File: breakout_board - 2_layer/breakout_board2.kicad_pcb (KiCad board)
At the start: 2 copper layers, 54 parts, among them J1 Conn_01x14, J2 Conn_01x14, J3 CONN_01X03, J4 CONN_02x04, J5 Conn_01x04, U1 TB6612FNG, U2 LP5907SNX-3.3/NOPB, U3 LSF0204RUTR, U4 ADP3330, U5 TLV70718PDQNR

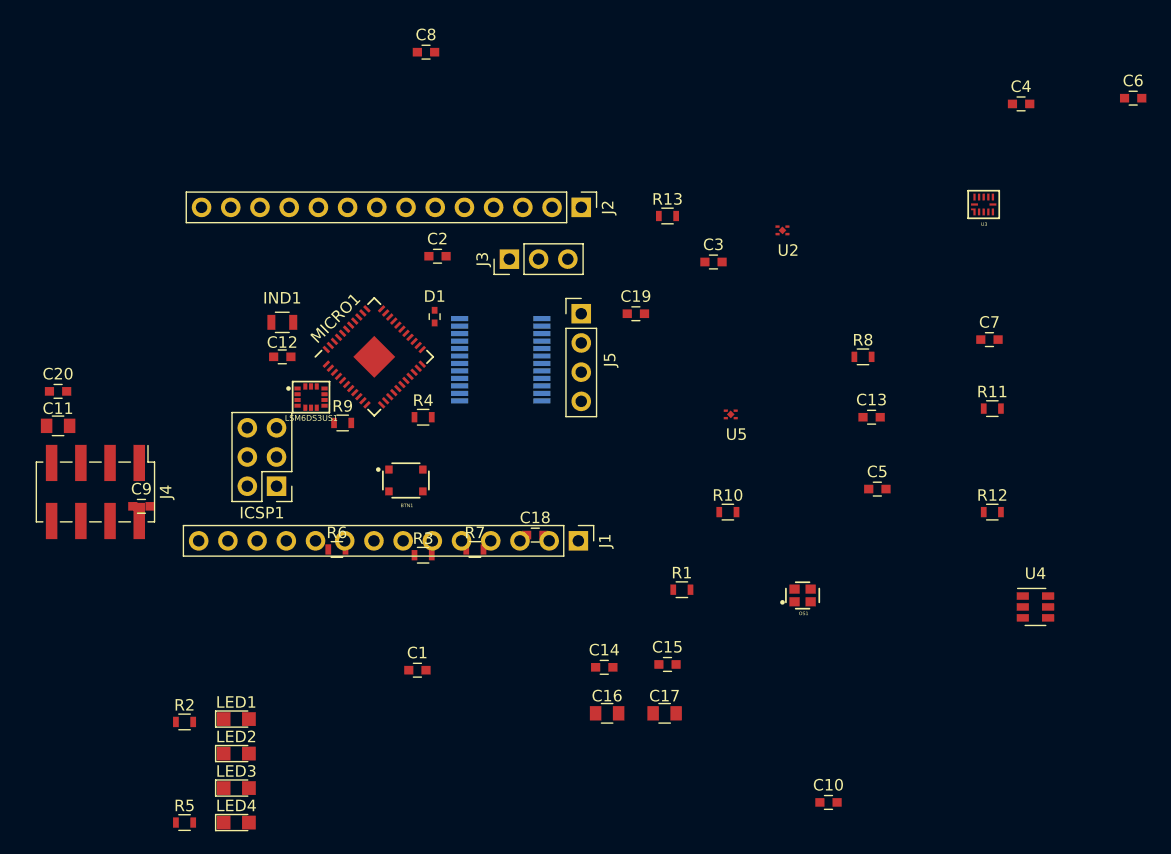
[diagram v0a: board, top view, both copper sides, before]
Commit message: Finished board v2
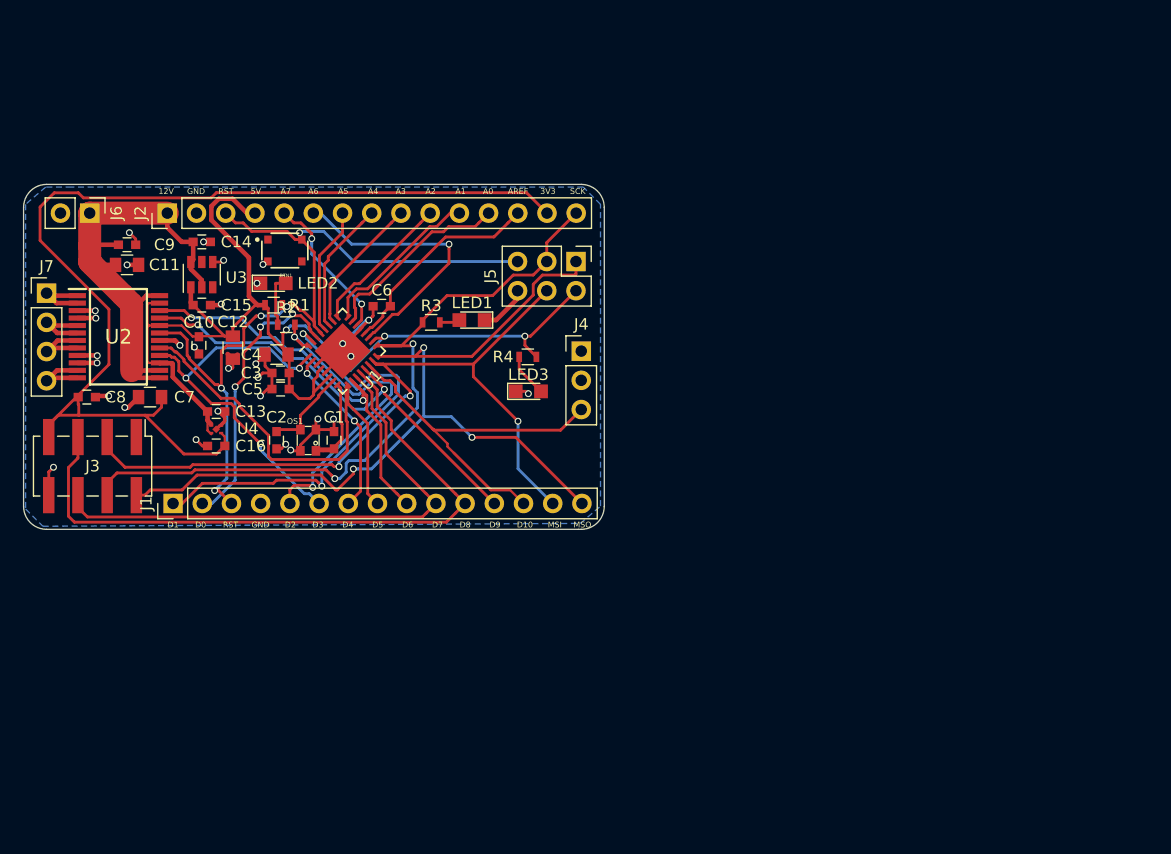
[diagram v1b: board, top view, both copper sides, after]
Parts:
- removed C17: 10uF, Capacitors_SMD:C_0805
- removed C18, C19, C20: 1uF, Capacitors_SMD:C_0603
- removed D1: CD1206-S01575, Capacitors_SMD:C_0402
- removed ICSP1: CONN_02X03, Pin_Headers:Pin_Header_Straight_2x03_Pitch2.54mm
- removed IND1: 30±25%ohm, Inductors_SMD:L_0805
- removed LED4: ON, LEDs:LED_0805
- removed LSM6DS3US1: IMU, footprints:LGA-14L
- removed MICRO1: ATMEGA32U4-MU, footprints:QFN-44-1EP_7x7mm_Pitch0.5mm_M
- removed R10, R11, R12, R13, R6, R7, R8, R9: 10K, Resistors_SMD:R_0603
- removed R5: 499, Resistors_SMD:R_0603
- removed U5: TLV70718PDQNR, footprints:DQN4
- added J6: Conn_01x02, Pin_Headers:Pin_Header_Straight_1x02_Pitch2.54mm, F.Cu at (92.8, 87.5)
- added J7: Conn_01x04, Pin_Headers:Pin_Header_Straight_1x04_Pitch2.54mm, F.Cu at (89.0, 94.5)
- C12, C8: value 1uF -> 10uF; footprint Capacitors_SMD:C_0603 -> Capacitors_SMD:C_0805
- C13, C14, C15: value 100nF -> 1uF
- C16: value 10uF -> 1uF; footprint Capacitors_SMD:C_0805 -> Capacitors_SMD:C_0603
- C4: value .1uF -> 4.7uF, 16V; footprint Capacitors_SMD:C_0603 -> Capacitors_SMD:C_0805
- C5: value .1uF -> 1uF
- C7, C9: value 1uF -> 100nF
- J1, J2: value Conn_01x14 -> Conn_01x15; footprint Pin_Headers:Pin_Header_Straight_1x14_Pitch2.54mm -> Pin_Headers:Pin_Header_Straight_1x15_Pitch2.54mm
- J3: value CONN_01X03 -> CONN_02x04; footprint Pin_Headers:Pin_Header_Straight_1x03_Pitch2.54mm -> Pin_Headers:Pin_Header_Straight_2x04_Pitch2.54mm_SMD
- J4: value CONN_02x04 -> CONN_01X03; footprint Pin_Headers:Pin_Header_Straight_2x04_Pitch2.54mm_SMD -> Pin_Headers:Pin_Header_Straight_1x03_Pitch2.54mm
- J5: value Conn_01x04 -> Conn_02x03_Odd_Even; footprint Pin_Headers:Pin_Header_Straight_1x04_Pitch2.54mm -> Pin_Headers:Pin_Header_Straight_2x03_Pitch2.54mm
- LED1: value RX -> RED
- LED2: value L -> GREEN
- LED3: value TX -> BLUE
- OS1: value 20MHZ -> 16MHZ; footprint footprints:ABM11AIG -> footprints:XC2119CT
- U1: value TB6612FNG -> ATMEGA328P-MUR; footprint footprints:SOP65P760X160-24N -> Housings_DFN_QFN:QFN-32-1EP_5x5mm_Pitch0.5mm; moved to F.Cu
- U2: value LP5907SNX-3.3/NOPB -> TB6612FNG; footprint footprints:DQN4 -> footprints:SOP65P760X160-24N
- U3: value LSF0204RUTR -> ADP3330; footprint footprints:R-PUQFN-N12 -> TO_SOT_Packages_SMD:SOT-23-6
- U4: value ADP3330 -> LP5907SNX-3.3/NOPB; footprint TO_SOT_Packages_SMD:SOT-23-6 -> footprints:DQN4
- moved C7 78.7 mm to (92.5, 103.5)
- moved U4 72.9 mm to (103.8, 106.3), turned to 180 degrees
- moved C4 68.3 mm to (109.0, 99.8)
- moved U3 68.3 mm to (102.5, 92.8), turned to 90 degrees
- moved C6 67.8 mm to (118.2, 95.6)
- moved C10 67.7 mm to (102.2, 99.0), turned to 270 degrees
- moved U2 58.5 mm to (95.2, 98.2)
- moved C13 57.0 mm to (103.8, 104.8)
- moved C5 52.6 mm to (109.3, 102.8)
- moved C15 51.2 mm to (102.5, 95.5)
- moved C14 50.9 mm to (102.5, 90.0)
- moved OS1 45.1 mm to (111.8, 107.2), turned to 90 degrees
- moved J4 44.0 mm to (135.5, 99.5), turned to 0 degrees
- moved R1 43.3 mm to (108.8, 95.5)
- moved LED3 42.8 mm to (130.9, 103.0)
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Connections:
- BTN1 pad 1: Net-(BTN1-Pad1) -> (no net)
- BTN1 pad 4: Net-(BTN1-Pad4) -> (no net)
- C10 pad 1: +3V3 -> +5V
- C11 pad 1: +3V3 -> +12V
- C13 pad 1: +1V8 -> +5V
- C16 pad 1: +12V -> +3V3
- C3 pad 1: Net-(C3-Pad1) -> GND
- C3 pad 2: GND -> +5V
- C4 pad 1: /AREF -> GND
- C4 pad 2: GND -> +5V
- C6 pad 2: +5V -> /AREF
- C7 pad 1: +12V -> +3V3
- C8 pad 1: Net-(C8-Pad1) -> +3V3
- C9 pad 1: +5V -> +12V
- J1 pad 1: /RESET -> /D1
- J1 pad 10: /D3/SCL -> /D7
- J1 pad 11: /D2/SDA -> /D8
- J1 pad 12: /IO11* -> /D9
- J1 pad 13: /MISO -> /D10
- J1 pad 14: /MOSI -> /D11/MOSI
- J1 pad 2: /IO10* -> /D0
- J1 pad 3: /IO9* -> /RESET
- J1 pad 4: /IO8 -> GND
- J1 pad 5: /IO12* -> /D2
- J1 pad 6: /D1/TX -> /D3
- J1 pad 7: /D0/RX -> /D4
- J1 pad 8: GND -> /D5
- J1 pad 9: /RESET -> /D6
- J2 pad 1: /IO13* -> +12V
- J2 pad 10: GND -> /A2
- J2 pad 11: /D7 -> /A1
- J2 pad 12: +12V -> /A0
- J2 pad 13: /RXLED/SS -> /AREF
- J2 pad 14: /SCK -> +3V3
- J2 pad 2: +5V -> GND
- J2 pad 3: /A0 -> /RESET
- J2 pad 4: /A1 -> +5V
- J2 pad 5: /A2 -> /A7
- J2 pad 6: /A3 -> /A6
- J2 pad 7: /A4 -> /A5
- J2 pad 8: /A5 -> /A4
- J2 pad 9: /AREF -> /A3
- J3 pad 1: GND -> (no net)
- J3 pad 2: Net-(J3-Pad2) -> /D12/MISO
- J3 pad 3: /D6* -> /D11/MOSI
- J4 pad 1: /IRQ -> GND
- J4 pad 2: /MISO -> (no net)
- J4 pad 3: /MOSI -> /D10
- J5 pad 1: /M2B -> /D12/MISO
- J5 pad 2: /M2A -> +5V
- J5 pad 3: /M1B -> /D13/SCK
- J5 pad 4: /M1A -> /D11/MOSI
- R2 pad 1: Net-(LED1-Pad2) -> Net-(LED2-Pad2)
- R2 pad 2: /RXLED/SS -> /D2
- R3 pad 1: Net-(LED2-Pad2) -> /D13/SCK
- R3 pad 2: /IO13* -> Net-(LED1-Pad2)
- R4 pad 2: /TXLED -> +5V
- U1 pad 1: /M2B -> /D3
- U1 pad 10: GND -> /D6
- U1 pad 11: /M1A -> /D7
- U1 pad 12: /M1A -> /D8
- U1 pad 13: +12V -> /D9
- U1 pad 14: +12V -> /D10
- U1 pad 15: +5V -> /D11/MOSI
- U1 pad 16: /D6* -> /D12/MISO
- U1 pad 17: /IO9* -> /D13/SCK
- U1 pad 18: GND -> +5V
- U1 pad 19: /RESET -> /A6
- U1 pad 2: /M2B -> /D4
- U1 pad 20: +5V -> /AREF
- U1 pad 21: /IO11* -> GND
- U1 pad 22: /IO10* -> /A7
- U1 pad 23: +5V -> /A0
- U1 pad 24: +12V -> /A1
- U1 pad 4: GND -> +5V
- U1 pad 5: /M2A -> GND
- U1 pad 6: /M2A -> +5V
- U1 pad 7: /M1B -> Net-(C2-Pad1)
- U1 pad 8: /M1B -> Net-(C1-Pad1)
- U1 pad 9: GND -> /D5
- U2 pad 1: +3V3 -> /M2B
- U2 pad 2: GND -> /M2B
- U2 pad 3: +5V -> GND
- U2 pad 4: +5V -> GND
- U2 pad 5: Net-(U2-Pad5) -> /M2A
- U3 pad 1: +1V8 -> +5V
- U3 pad 2: /SCL_1V8 -> +12V
- U3 pad 3: /SDA_1V8 -> (no net)
- U3 pad 4: /INT1 -> GND
- U3 pad 5: /INT2 -> (no net)
- U3 pad 6: GND -> +12V
- U4 pad 1: +5V -> +3V3
- U4 pad 2: +12V -> GND
- U4 pad 3: Net-(U4-Pad3) -> +5V
- U4 pad 4: GND -> +5V
- U4 pad 5: Net-(U4-Pad5) -> GND
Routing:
- net +5V: track 0.00 -> 102.7 mm, vias 0 -> 3
- net +3V3: track 0.00 -> 93.3 mm
- net /D12/MISO: track 0.00 -> 75.1 mm, vias 0 -> 3
- net /RESET: track 0.00 -> 73.5 mm, vias 0 -> 5
- net GND: track 0.00 -> 68.5 mm, vias 0 -> 30
- net /D11/MOSI: track 0.00 -> 68.3 mm, vias 0 -> 3
- net /D13/SCK: track 0.00 -> 64.2 mm, vias 0 -> 2
- net /D8: track 0.00 -> 57.8 mm
- net /D7: track 0.00 -> 46.9 mm
- net +12V: track 0.00 -> 42.8 mm
- net /D9: track 0.00 -> 40.0 mm, vias 0 -> 2
- net /D5: track 0.00 -> 39.2 mm
- net /D1: track 0.00 -> 38.3 mm, vias 0 -> 2
- net /D6: track 0.00 -> 35.8 mm, vias 0 -> 2
- net /D3: track 0.00 -> 33.8 mm, vias 0 -> 3
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- added copper zone on B.Cu, net GND
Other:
- board outline added: 50.5 x 30 mm
- net class Wide added: clearance 0.2, trace_width 0.4, via_dia 0.6, via_drill 0.4
- board text added: "12V"
- board text added: "3V3"
- board text added: "5V"
- board text added: "A0"
- board text added: "A1"
- board text added: "A2"
- board text added: "A3"
- board text added: "A4"
- board text added: "A5"
- board text added: "A6"
- board text added: "A7"
- board text added: "AREF"
- board text added: "COMBATBOARD V1.0 ARPAN RAU"
- board text added: "D0"
- board text added: "D1"
- board text added: "D10"
- board text added: "D2"
- board text added: "D3"
- board text added: "D4"
- board text added: "D5"
- board text added: "D6"
- board text added: "D7"
- board text added: "D8"
- board text added: "D9"
- board text added: "GND"
- board text added: "MSI"
- board text added: "MSO"
- board text added: "RST"
- board text added: "SCK"
